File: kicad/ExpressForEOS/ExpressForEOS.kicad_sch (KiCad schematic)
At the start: 17 parts, among them J1 Conn_02x17_Counter_Clockwise, U1 74HC4051, U10 74LS08, U11 74LS156, U12 74LS156, U13 74LS373, U14 ICM7218BIPI, U15 MAX150BCPP, U16 LM358, U2 74HC4051, U3 74HC4051, U4 74HC4051, U5 CD4066BE, U6 74LS138, U7 74LS374, U8 74LS374, U9 74LS245

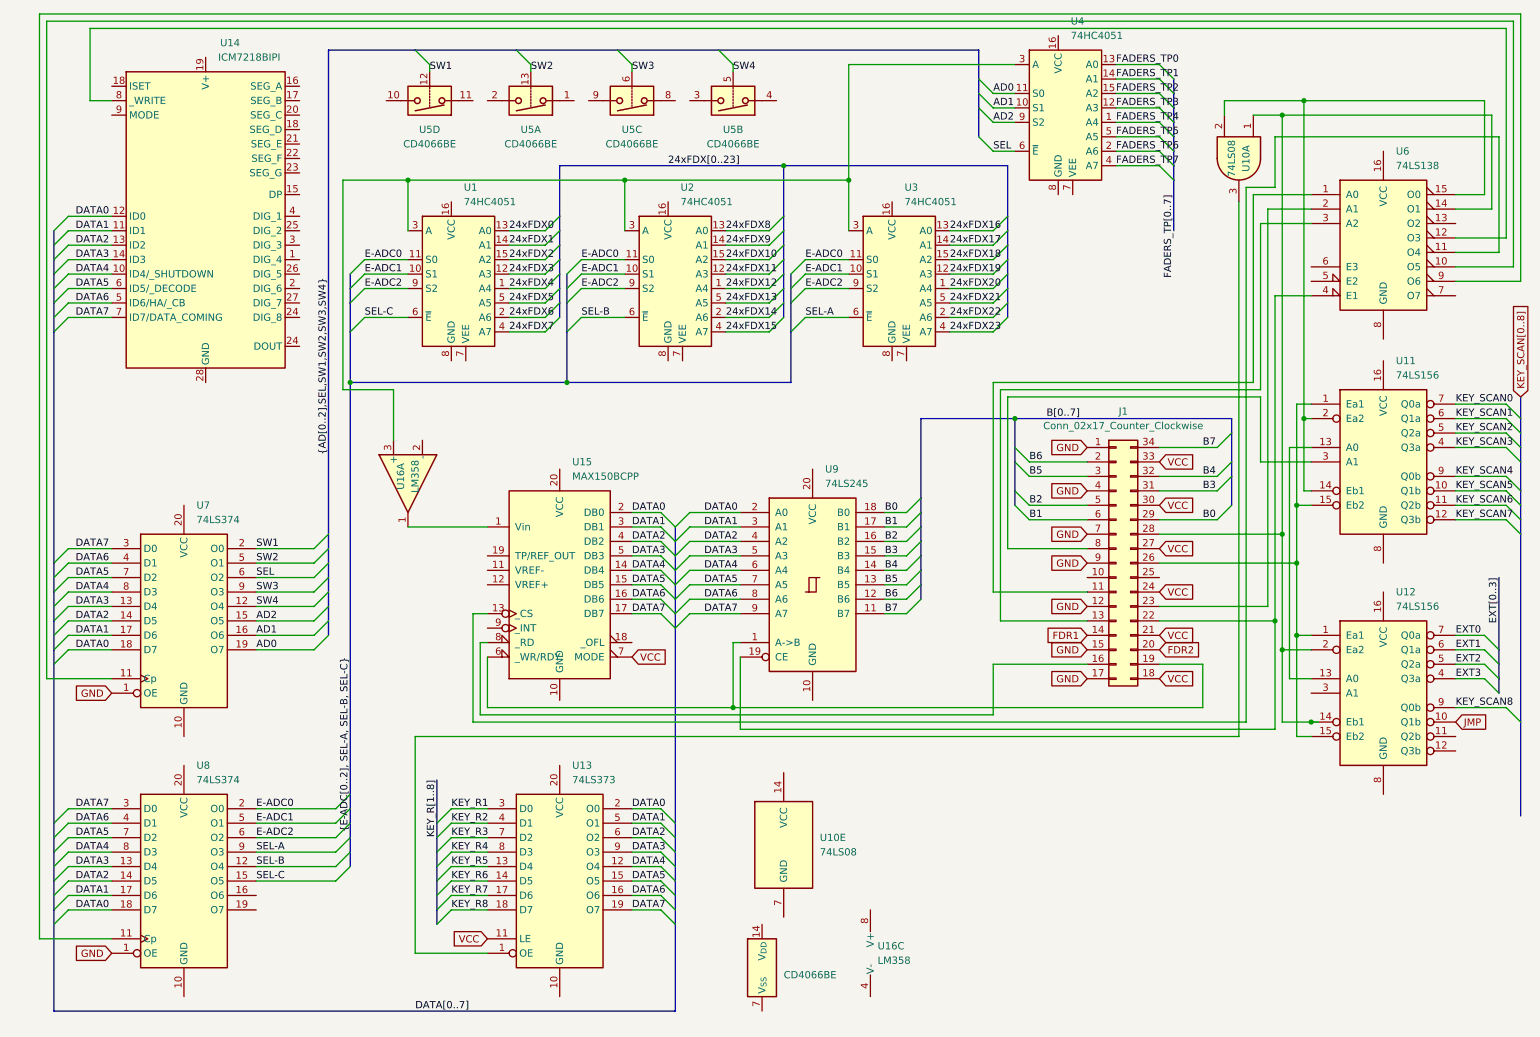
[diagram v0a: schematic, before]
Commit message: Schem update
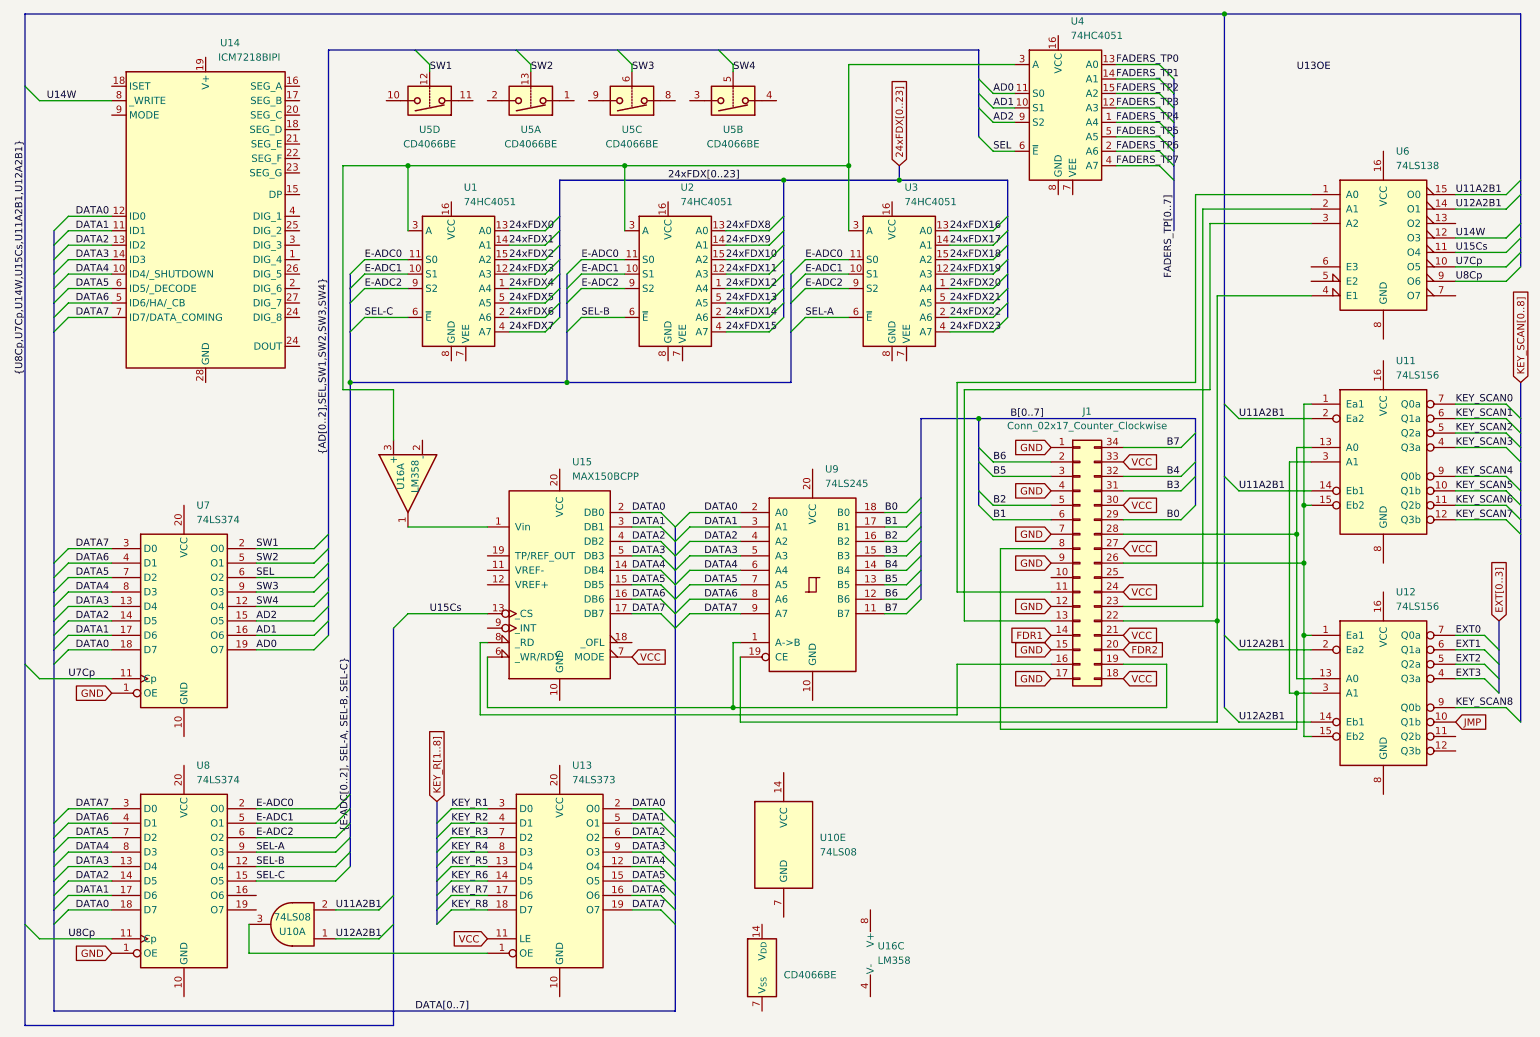
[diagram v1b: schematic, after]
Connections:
- net at U11.13 (A0), U12.13 (A0): now also J1.28 (Pin_28)
- net U11A2B1: now reaches U10.2, U11.14 (Eb1), U11.2 (Ea2), U6.15 (O0)
- net at J1.8 (Pin_8), U11.3 (A1): now also U12.3 (A1)
- net U8Cp: now reaches U6.9 (O6), U8.11 (Cp)
- net U14W: now reaches U14.8 (_WRITE), U6.12 (O3)
- net U7Cp: now reaches U6.10 (O5), U7.11 (Cp)
- net U15Cs: now reaches U15.13 (_CS), U6.11 (O4)
- net U12A2B1: now reaches U10.1, U12.14 (Eb1), U12.2 (Ea2), U6.14 (O1)
- net U12A2B1: no longer J1.28 (Pin_28)
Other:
- moved on the sheet: J1, U10A
